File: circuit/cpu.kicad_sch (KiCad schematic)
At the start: 28 parts, among them J1 Port B, J2 Port C, J3 Port E, J3 Port F, J4 Port A, J43 Port G, J5 Port D, J50 External button, U1 74HTC138, U6 74LS08, U8 74LS125

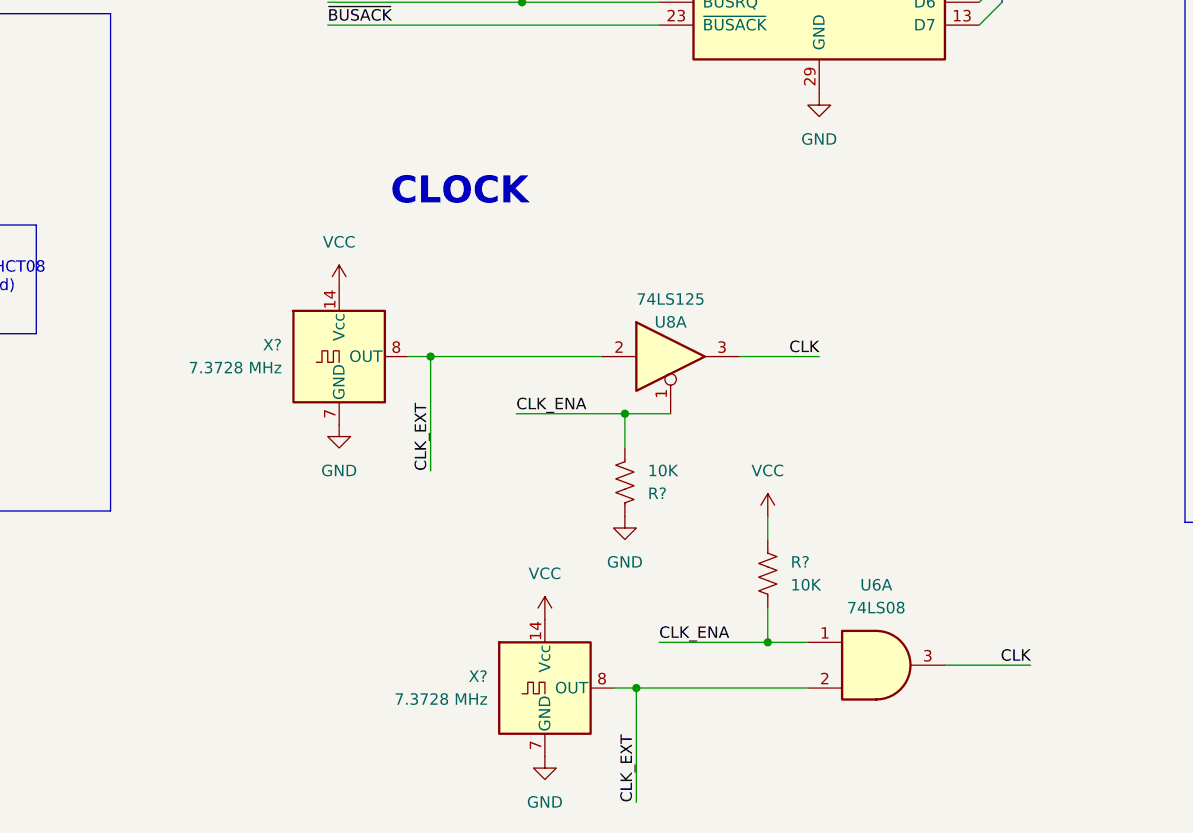
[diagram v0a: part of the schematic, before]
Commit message: .
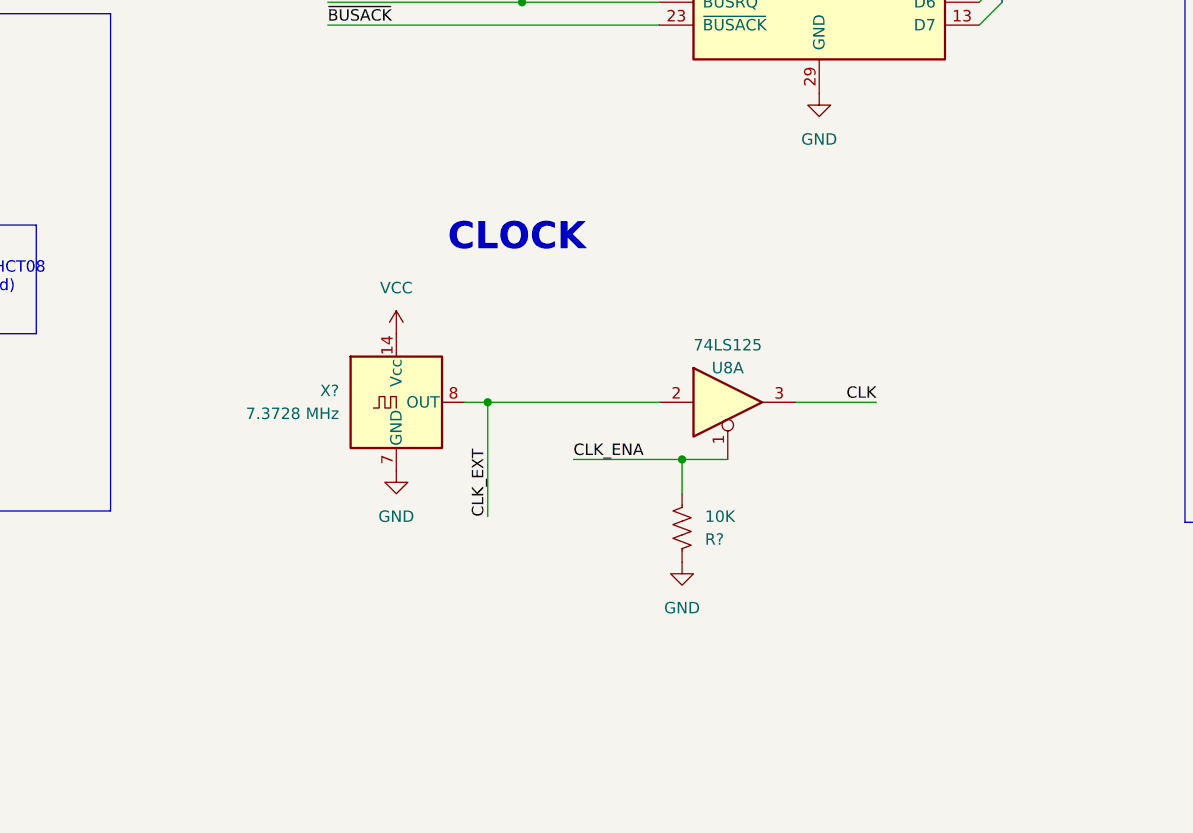
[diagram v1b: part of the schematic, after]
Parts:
- removed R?: 10K, symbol Device:R_US
- removed U6: 74LS08, symbol 74xx:74LS08
- removed X?: 7.3728 MHz, Oscillator:Oscillator_DIP-14, symbol Oscillator:ACO-xxxMHz
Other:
- moved on the sheet: R?, U8A, X?
